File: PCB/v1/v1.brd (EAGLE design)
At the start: 59 x 39 mm, 63 parts, among them U2 AT24C512C-SHD-B

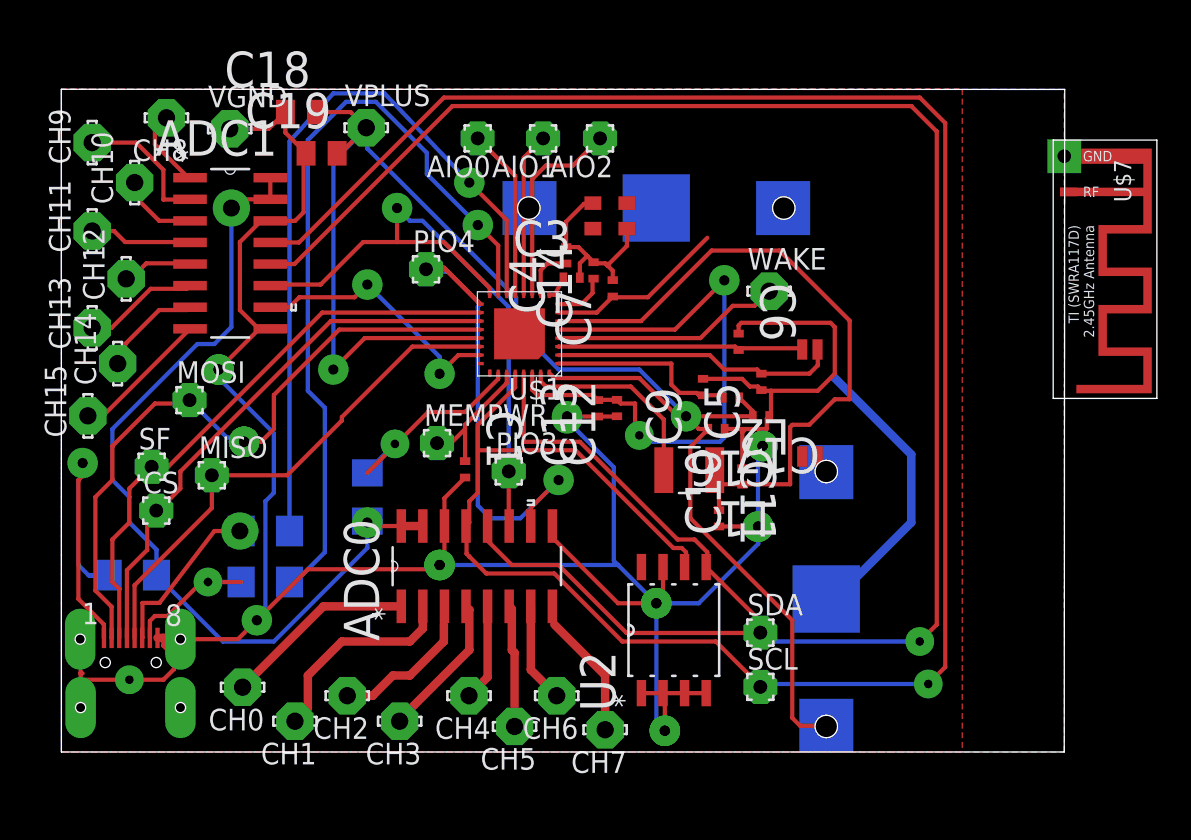
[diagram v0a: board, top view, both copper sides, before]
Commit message: latest
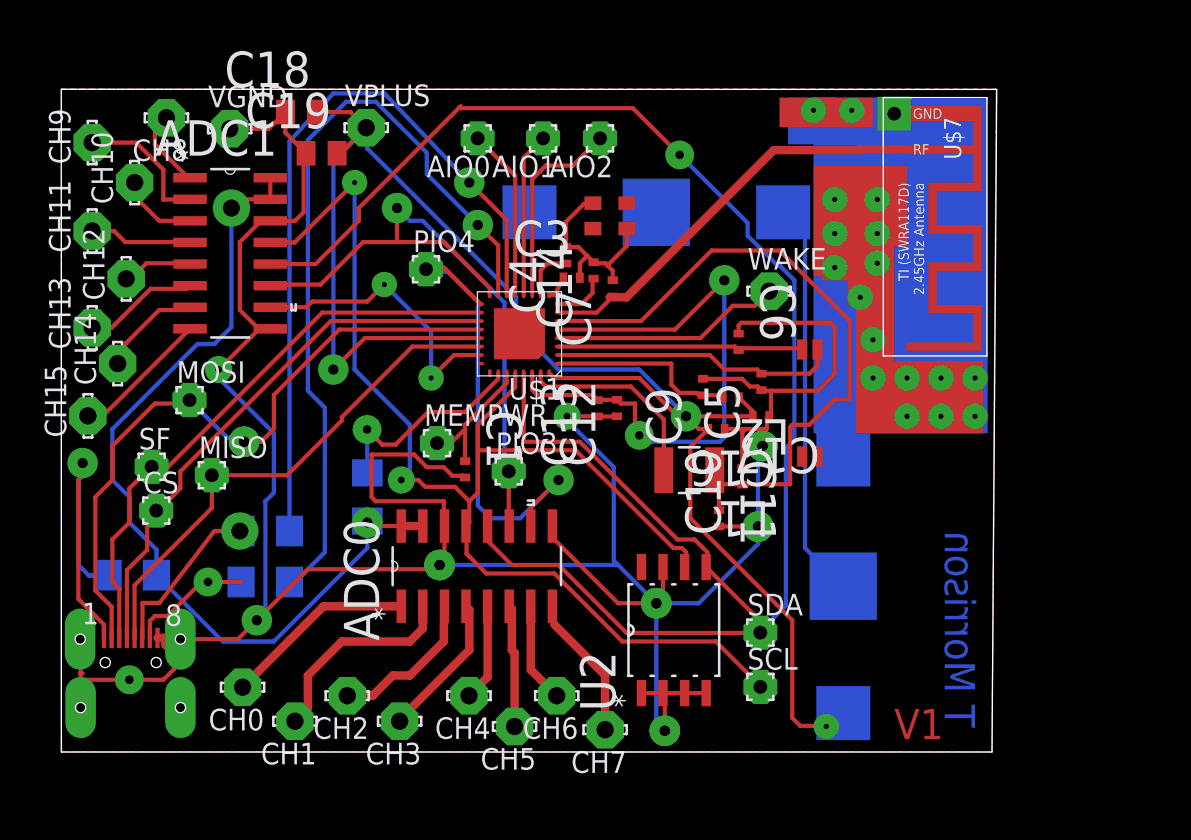
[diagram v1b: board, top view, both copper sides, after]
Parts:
- moved U$5 24.9 mm to (35.0, 31.8), turned to 0 degrees
- moved U$6 24.8 mm to (46.0, 9.75), turned to 90 degrees
- moved U$7 10.3 mm to (48.8, 38.0)
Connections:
- net GND: now also U$5.NEG; no longer U$6.NEG
- net N$34: now also U$6.POS@1; no longer U$5.POS@1
- net N$48: now also U$5.POS@1, U$6.NEG; no longer U$5.NEG, U$6.POS@1
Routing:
- net N$21: track 135.9 -> 78.5 mm, vias 1 -> 2
- net N$22: track 126.4 -> 104.2 mm
- net N$76: track 0.00 -> 20.4 mm
- net GND: track 182.6 -> 193.7 mm
- net N$48: track 17.3 -> 24.8 mm
- net N$74: track 7.20 -> 0.00 mm
- net N$34: track 98.7 -> 100.0 mm
- net N$24: track 16.1 -> 17.4 mm
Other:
- board size 59 x 39 mm -> 55 x 39 mm
- board text added: "T Morrison"
- board text added: "V1"
